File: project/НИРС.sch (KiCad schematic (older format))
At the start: 32 parts, among them IC101 AT24C64A-10PU-2.7, J10 J10, J7 J7, J8 J8, J9 J9, j6 J6

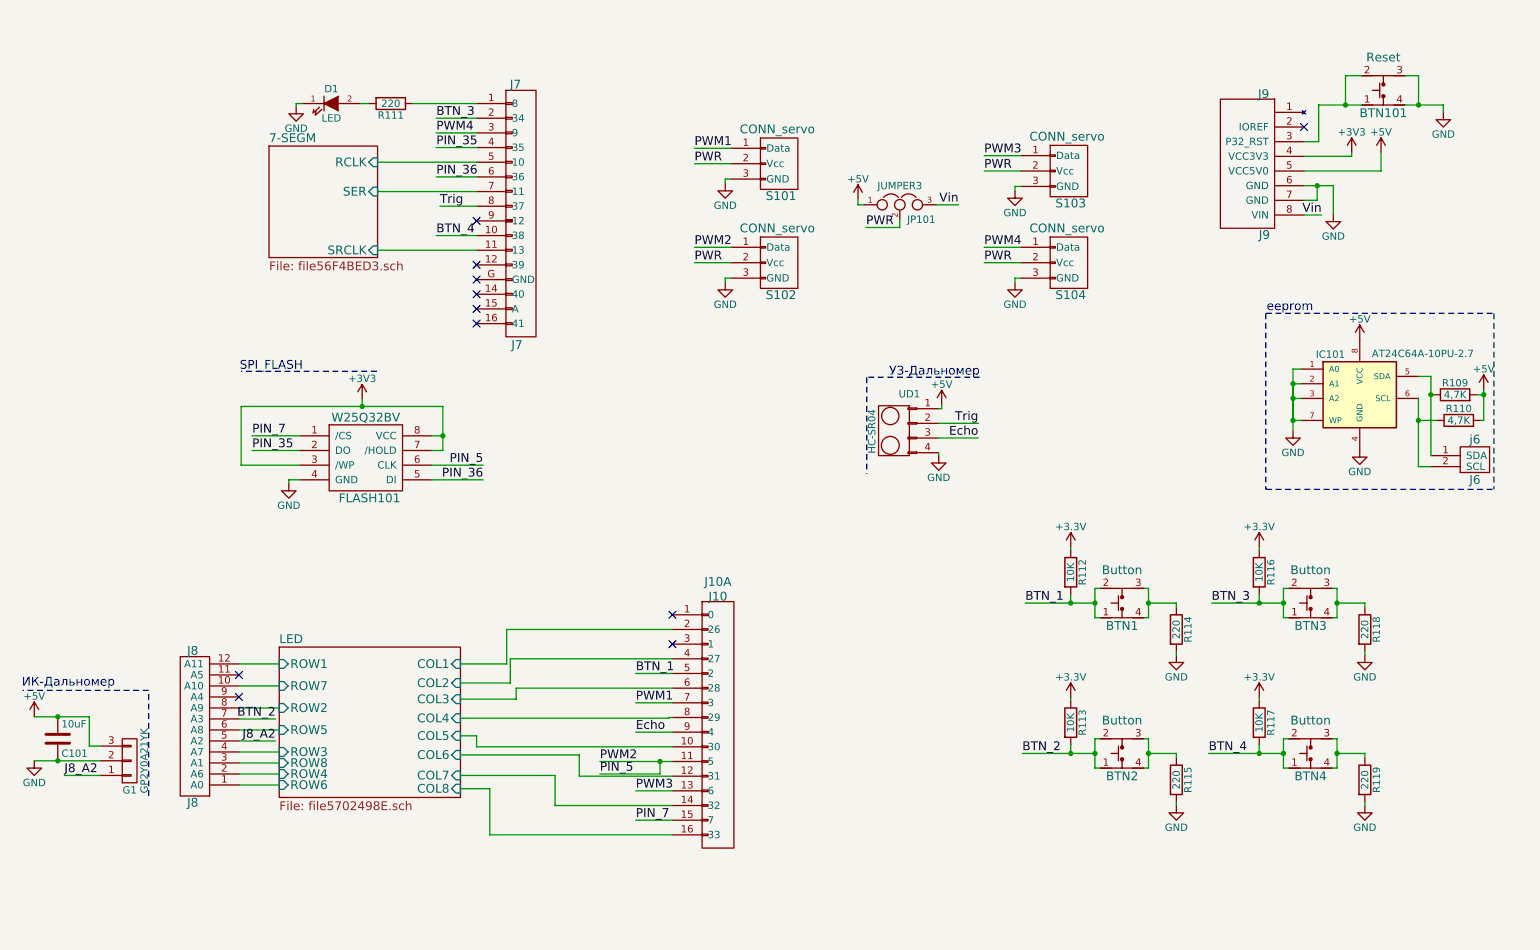
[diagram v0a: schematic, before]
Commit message: Add files via upload
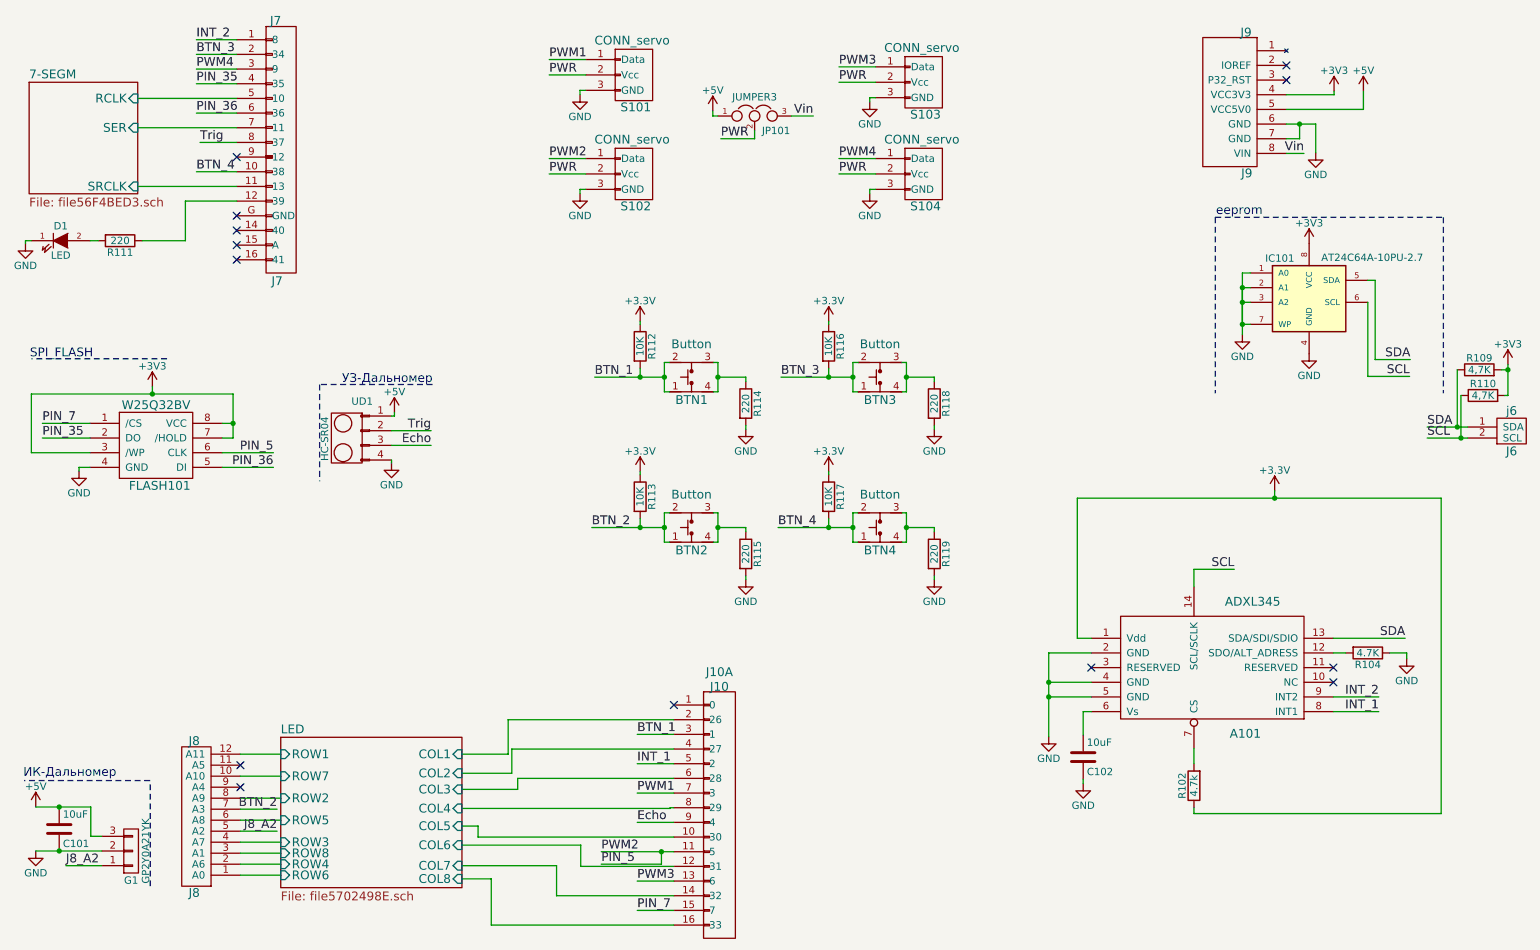
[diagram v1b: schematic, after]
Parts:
- removed BTN101: Reset, WIFIRE:RESET, symbol Reset
- added A101: ADXL345, WIFIRE:ADXL345, symbol ADXL345
- added C102: 10uF, Capacitors_SMD:C_0805, symbol C
- added R102: 4.7k, Resistors_SMD:R_0805, symbol R
- added R104: 4.7K, Resistors_SMD:R_0805, symbol R
- IC101: footprint Housings_DIP:DIP-8_W7.62mm -> WIFIRE:JEDEC_SOIC
- UD1: footprint WIFIRE:HC-SR04 -> Pin_Headers:Pin_Header_Straight_1x04
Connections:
- net +3V3: now also IC101.8 (VCC), R109.2, R110.2, A101.1 (Vdd), R102.1
- net +5V: no longer IC101.8 (VCC), R109.2, R110.2
- net BTN_1: now also J10.3 (1); no longer J10.5 (2)
- net GND: now also A101.2 (GND), A101.4 (GND), A101.5 (GND), C102.1, R104.1
- net at R111.1: now also J7.12 (39); no longer J7.1 (8)
- net SDA: now reaches IC101.5 (SDA), R109.1, j6.1 (SDA)
- net SDA: now also A101.13 (SDA/SDI/SDIO)
- net SCL: now reaches IC101.6 (SCL), R110.1, j6.2 (SCL)
- net SCL: now also A101.14 (SCL/SCLK)
- new net: A101.12 (SDO/ALT_ADRESS), R104.2
- new net: A101.6 (Vs), C102.2
- new net: A101.7 (CS), R102.2
- new net INT_1: A101.8 (INT1), J10.5 (2)
- new net INT_2: A101.9 (INT2), J7.1 (8)
- no-connect marks 11 -> 13
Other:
- moved on the sheet: BTN1, BTN2, BTN3, BTN4, C101, D1, FLASH101, G1, IC101, J10A, J7, J8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
